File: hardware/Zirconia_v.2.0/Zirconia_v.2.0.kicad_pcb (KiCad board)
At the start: 2 copper layers, 39 x 91 mm, 91 parts, among them J1 BD125-10-A-0305-0580-L-B, J2 Conn_01x04, J4 BD125-10-A-0305-0580-L-B, P1 Red, P2 Blk, P3 Red, P4 Blk, P6 PicoBlade_53047-0210, Q1 LTR, Q2 LTR, Q3 LTR, Q4 LTR, Q5 IRLML6344, Q6 IRLML6344, Q7 IRLML6344, Q8 IRLML6344, Q9 DMC2400UV-7, SW1 KMR211NG LFS, SW2 SS12D01G4, U1 MA302/MA730, U10 ENCODER_CONNECT_IC, U11 LP5907MFX-3.0, U12 STLINK-V3MOS, U2 ENCODER_CONNECT_IC, U3 DRV8836DSSR, U4 STM32F411CEU6/STM32F413CHU6, U5 ENCODER_CONNECT_PCB, U6 ENCODER_CONNECT_PCB, U7 MCP73831T-2ACI/OT, U8 ICM-42688-P, U9 MA302/MA730

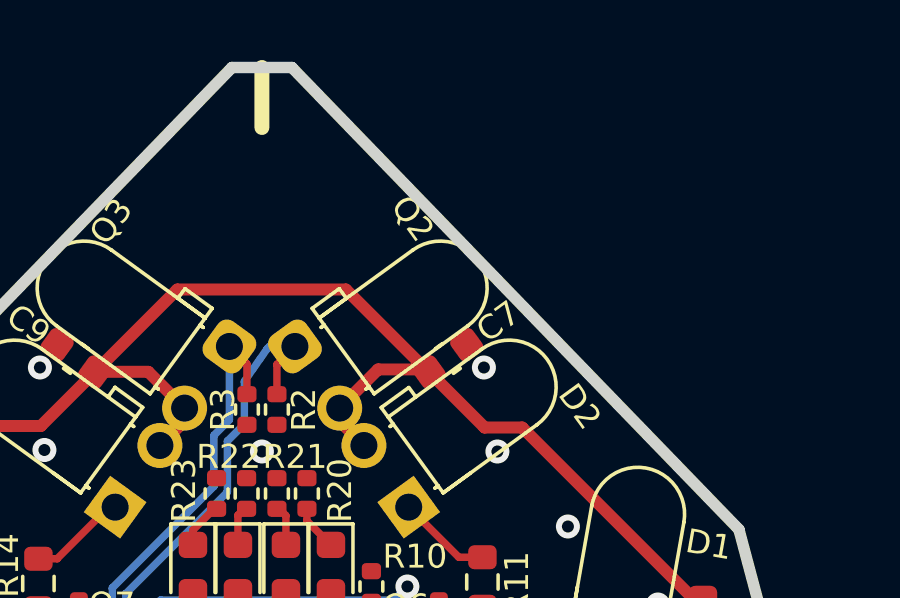
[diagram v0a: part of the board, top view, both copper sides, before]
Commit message: update
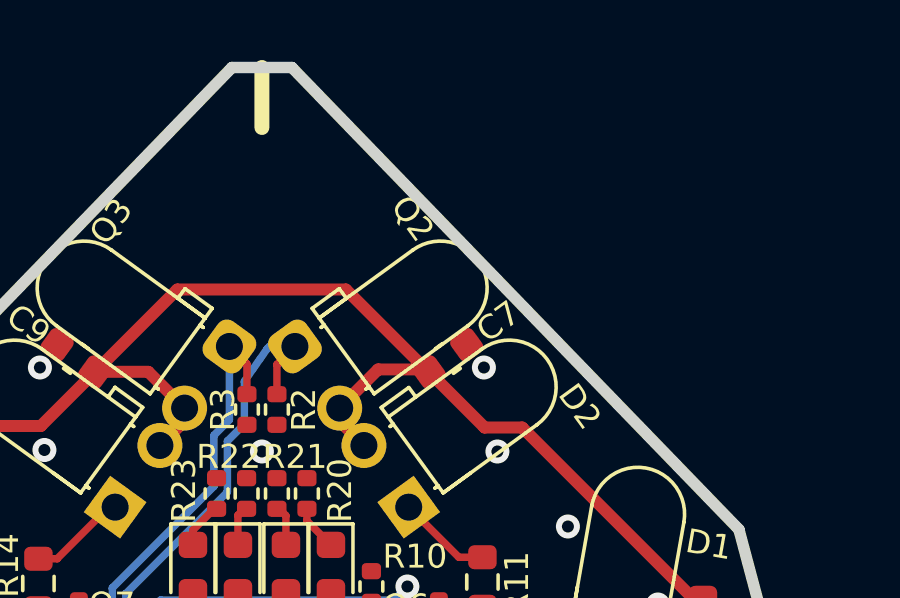
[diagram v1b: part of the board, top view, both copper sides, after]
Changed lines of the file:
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@@
 		(fp_arc
 			(start 0.29 5.07)
-			(mid -1.269999 6.629999)
+			(mid -1.270001 6.63)
 			(end -2.83 5.07)
 			(stroke
@@
 		(fp_arc
 			(start 0.23 5.07)
-			(mid -1.27 6.569999)
+			(mid -1.27 6.57)
 			(end -2.77 5.07)
 			(stroke
@@
 		(fp_arc
 			(start 2.83 5.07)
-			(mid 1.27 6.629999)
+			(mid 1.27 6.629998)
 			(end -0.290001 5.07)
 			(stroke
